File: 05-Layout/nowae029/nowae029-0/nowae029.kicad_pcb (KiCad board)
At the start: 2 copper layers, 100 x 99.9 mm, 168 parts, among them P101 COMM_3, P102 SUPPLY_3, P103 COMM_4, P104 SUPPLY_4, P201 DEBUG, P401 BATTERY, P501 632722110112, P502 UART, Q701 BCW68GLT1G, U201 STM32L073CBT6, U301 TCA9554PWR, U302 TCA9554PWR, U401 TLV70233DBV, U501 FT230XS, U601 TCA9554PWR, U602 TCA9554PWR, Y201 32768

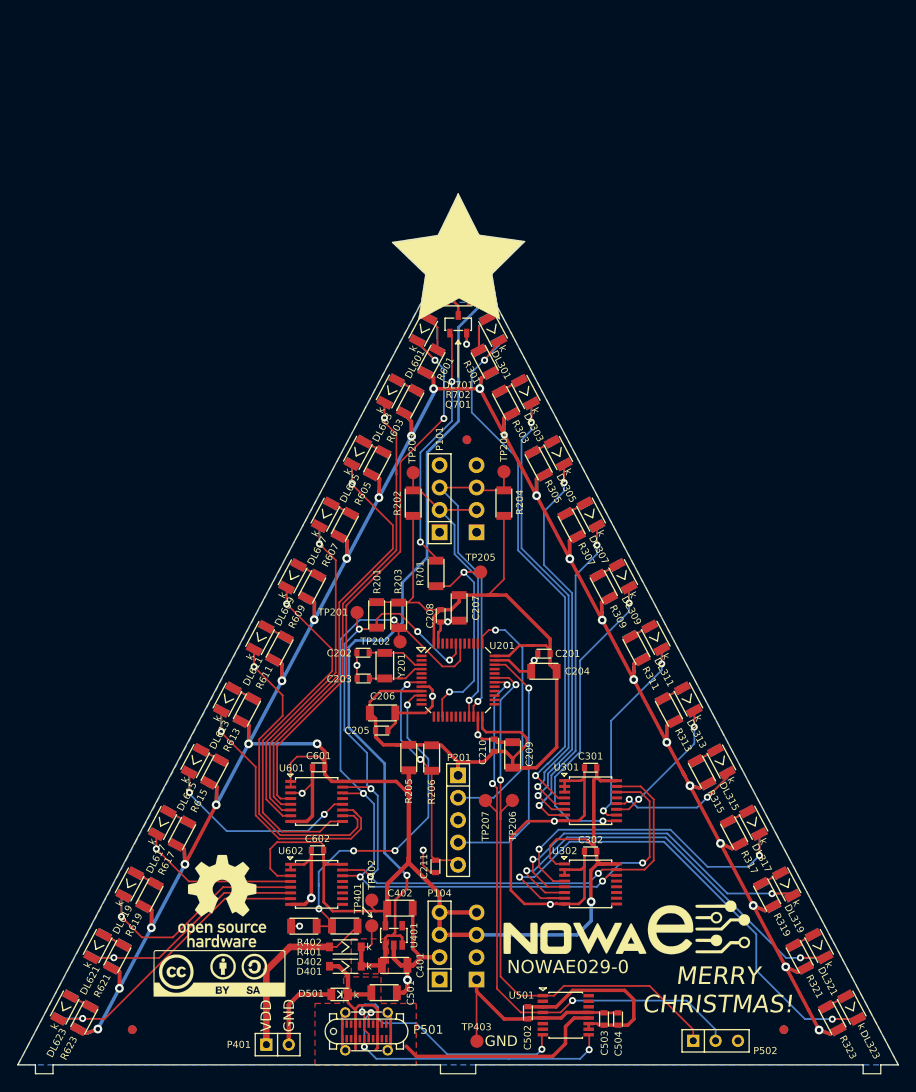
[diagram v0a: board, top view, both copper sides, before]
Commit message: small fix
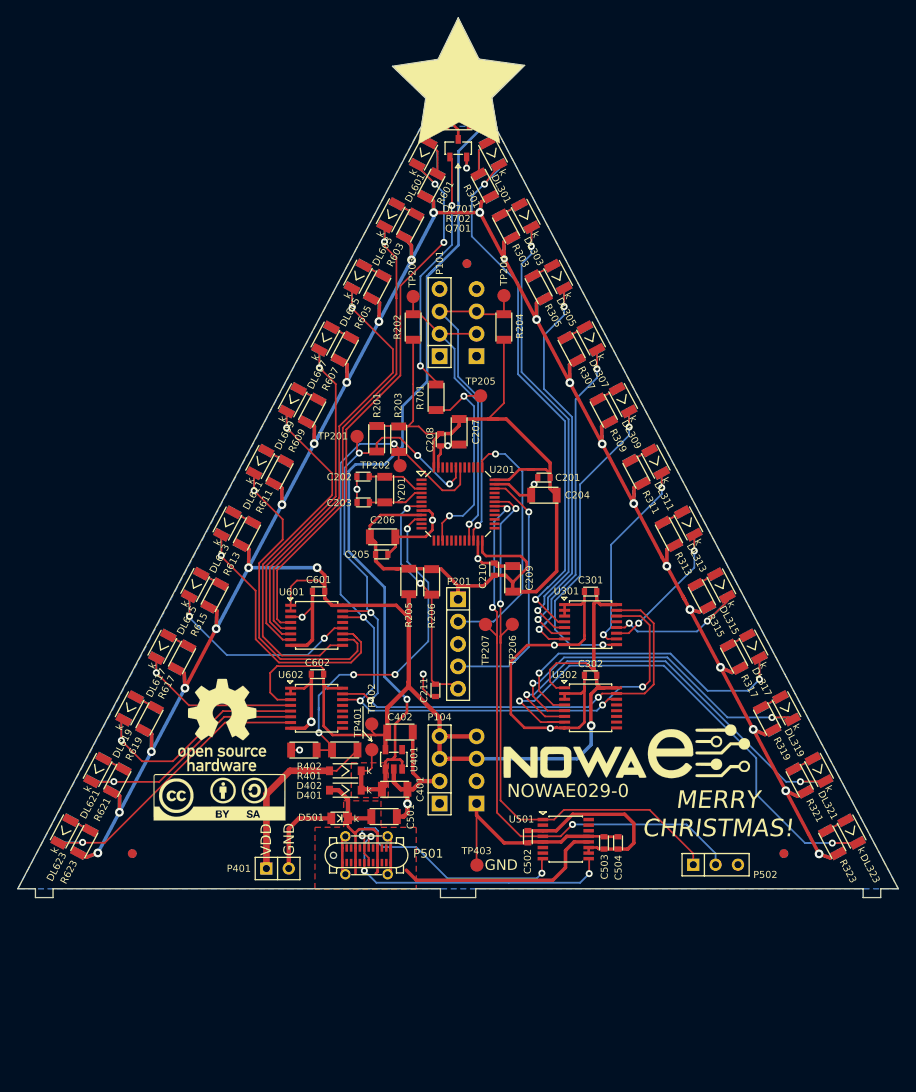
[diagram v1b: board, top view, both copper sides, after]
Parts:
- moved C501 20.0 mm to (91.6, 120.8)
- moved D401 20.0 mm to (87.2, 117.8)
- moved DL620 20.0 mm to (62.7, 108.5)
- moved DL623 20.0 mm to (55.3, 122.5)
- moved R619 20.0 mm to (65.0, 109.7)
- moved R620 20.0 mm to (65.0, 109.7)
- moved TP401 20.0 mm to (90.2, 113.2)
- moved U401 20.0 mm to (92.7, 114.3)
- moved U501 20.0 mm to (112.2, 123.4)
- moved DL301 20.0 mm to (104.0, 45.5)
- moved DL305 20.0 mm to (111.4, 59.5)
- moved DL306 20.0 mm to (111.4, 59.5)
- moved DL602 20.0 mm to (96.0, 45.5)
- moved DL603 20.0 mm to (92.3, 52.5)
- moved DL604 20.0 mm to (92.3, 52.5)
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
